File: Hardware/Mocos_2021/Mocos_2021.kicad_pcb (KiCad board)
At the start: 2 copper layers, 124.5 x 24.9 mm, 104 parts, among them IC1 TC2117, J1 USB_B_Mini, J2 SERIAL PORT, J3 Programming, Q1 IRFS7530, Q2 IRFS7530, Q3 IRFS7530, Q4 IRFS7530, Q5 IRFS7530, Q6 IRFS7530, U1 DRV8302, U2 STM32F40X_LQFP64, X1 8MHz, 10ppm

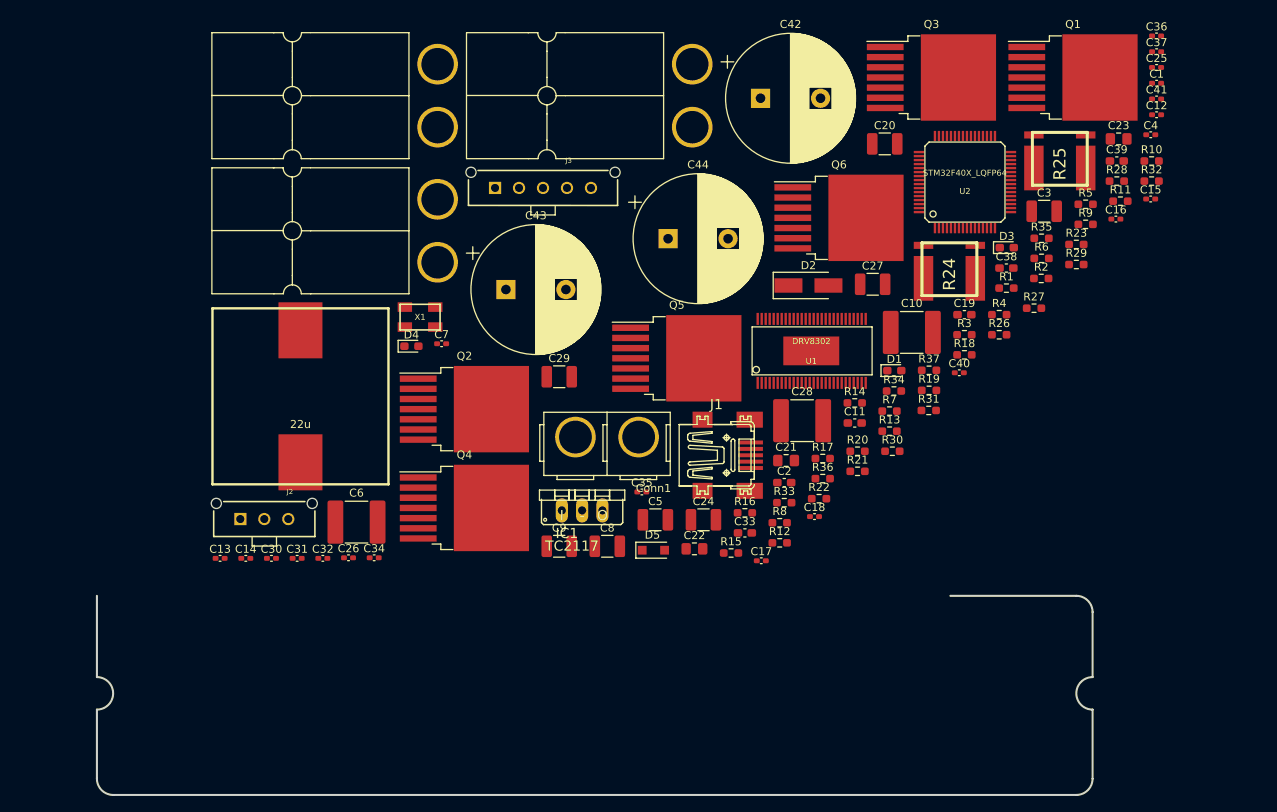
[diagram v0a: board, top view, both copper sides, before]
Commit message: Finished STM32 Layout
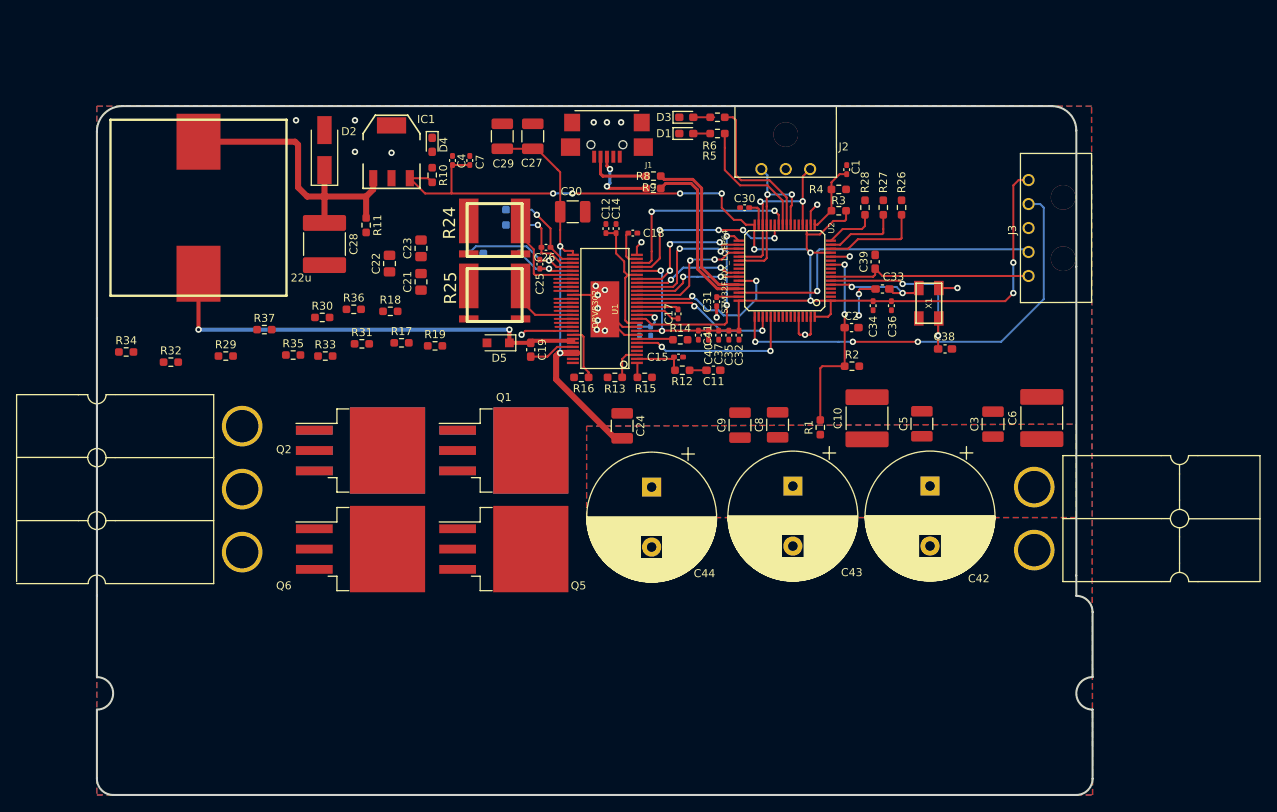
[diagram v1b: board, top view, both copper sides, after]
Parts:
- removed Conn3: Phase2, MRDT_Connectors:Anderson_2_Horizontal_Side_by_Side
- removed Conn4: Phase3, MRDT_Connectors:Anderson_2_Horizontal_Side_by_Side
- removed R7: 0, Resistor_SMD:R_0603_1608Metric_Pad0.98x0.95mm_HandSolder
- C1: value 2.2u -> 2.2u 16V
- C11: value 6.8n -> 6.8n, 50V
- C13, C16: moved to B.Cu
- C17: value 22n -> 22n, 50V
- C2, C39: value 100n -> 100n, 50V
- C38: value 15p -> 15p, 50V
- C4: value 2.2u -> 2.2u, 6V
- C7: value 100u -> 100u, 6V
- Conn1: footprint MRDT_Connectors:Anderson_2_Vertical_Sidy_by_Side -> MRDT_Connectors:Anderson_2_Horizontal_Side_by_Side_PV
- Conn2: value Phase1 -> Phases; footprint MRDT_Connectors:Anderson_2_Horizontal_Side_by_Side -> MRDT_Connectors:Anderson_3_Horizontal_Side_by_Side
- IC1: footprint v-reg-78XXS -> crf1:SOT-223
- J1: footprint crf1:mini_USB_gnd -> crf1:USB-UX60R-MB-5ST
- J2: footprint MRDT_Connectors:MOLEX_uF_S_03_Vertical -> MRDT_Connectors:MOLEX_uF_S_03_Horizontal
- J3: footprint MRDT_Connectors:MOLEX_uF_S_05_Vertical -> MRDT_Connectors:MOLEX_uF_S_05_Horizontal
- Q1, Q2, Q5, Q6: value IRFS7530 -> IRFZ44ESTRLPBF; footprint Package_TO_SOT_SMD:TO-263-7_TabPin4 -> Package_TO_SOT_SMD:TO-263-3_TabPin4
- Q3, Q4: value IRFS7530 -> IRFZ44ESTRLPBF; footprint Package_TO_SOT_SMD:TO-263-7_TabPin4 -> Package_TO_SOT_SMD:TO-263-3_TabPin4; moved to B.Cu
- R20, R21, R22, R23: value 100K -> 100; moved to B.Cu
- moved R32 124.7 mm to (73.8, 101.2)
- moved R29 106.9 mm to (80.6, 100.5)
- moved R34 96.1 mm to (68.2, 99.9)
- moved R35 94.7 mm to (89.1, 100.3)
- moved R11 94.3 mm to (98.2, 84.1), turned to 270 degrees
- moved R10 89.9 mm to (106.4, 77.8), turned to 90 degrees
- moved C23 88.3 mm to (105.0, 87.0), turned to 90 degrees
- moved C4 87.3 mm to (109.0, 76.0), turned to 90 degrees
- moved C6 86.6 mm to (182.6, 108.2), turned to 90 degrees
- moved Q1 85.1 mm to (115.4, 112.3)
- moved R37 83.2 mm to (85.4, 97.2)
- moved C25 80.9 mm to (119.9, 89.0), turned to 270 degrees
- moved J2 77.9 mm to (150.6, 78.1)
- moved R25 73.7 mm to (114.2, 94.7), turned to 180 degrees
- moved C30 73.6 mm to (145.5, 81.9)
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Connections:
- net USB_DM renamed USB-
- net USB_DP renamed USB+
- Conn2 pad 1: H2_LOW -> H1_VS
- Conn2 pad 2: (no net) -> H2_VS
- X1 pad 2: Net-(C38-Pad1) -> H2_LOW
- X1 pad 3: H2_LOW -> Net-(C38-Pad1)
- X1 pad 4: (no net) -> H2_LOW
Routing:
- net +3V3: track 0.00 -> 167.0 mm, vias 0 -> 11
- net Net-(C19-Pad1): track 0.00 -> 56.2 mm, vias 0 -> 2
- net Net-(J3-Pad2): track 0.00 -> 55.0 mm, vias 0 -> 3
- net VDD: track 0.00 -> 50.4 mm, vias 0 -> 2
- net Net-(J3-Pad4): track 0.00 -> 41.5 mm, vias 0 -> 1
- net +5V: track 0.00 -> 39.4 mm
- net H2_LOW: track 0.00 -> 37.4 mm, vias 0 -> 22
- net Net-(C39-Pad1): track 0.00 -> 26.0 mm
- net BR_SO2: track 0.00 -> 25.4 mm, vias 0 -> 2
- net DC_CAL: track 0.00 -> 24.2 mm, vias 0 -> 2
- net AN_IN: track 0.00 -> 24.1 mm, vias 0 -> 2
- net Net-(C38-Pad1): track 0.00 -> 23.8 mm, vias 0 -> 2
- net BR_SO1: track 0.00 -> 23.3 mm, vias 0 -> 4
- net TX_SDA_NSS: track 0.00 -> 22.5 mm, vias 0 -> 2
- net RX_SCL_MOSI: track 0.00 -> 22.0 mm, vias 0 -> 2
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- added copper zone on B.Cu, net H2_LOW
- added copper zone on F.Cu, net H2_LOW
- added copper zone on B.Cu, net VDD
- added copper zone on F.Cu, net VDD
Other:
- board size 124.5 x 24.9 mm -> 124.5 x 86.1 mm
